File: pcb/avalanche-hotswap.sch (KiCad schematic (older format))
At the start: 107 parts, among them J1 TRRS, J2 LED, J3 OLED, P1 i2c_pin, P2 i2c_pin, SW1 SW_Push, SW10 SW_Push, SW11 SW_Push, SW12 SW_Push, SW13 SW_Push, SW14 SW_Push, SW15 SW_Push, SW16 SW_Push, SW17 SW_Push, SW18 SW_Push, SW19 SW_Push, SW2 SW_Push, SW20 SW_Push, SW21 SW_Push, SW22 SW_Push, SW23 SW_Push, SW24 SW_Push, SW25 SW_Push, SW26 SW_Push, SW27 SW_Push, SW28 SW_Push, SW29 SW_Push, SW3 SW_Push, SW30 SW_Push, SW31 SW_Push, SW32 SW_Push, SW4 SW_Push, SW5 SW_Push, SW6 SW_Push, SW7 SW_Push, SW8 SW_Push, SW9 SW_Push, U1 ProMicro

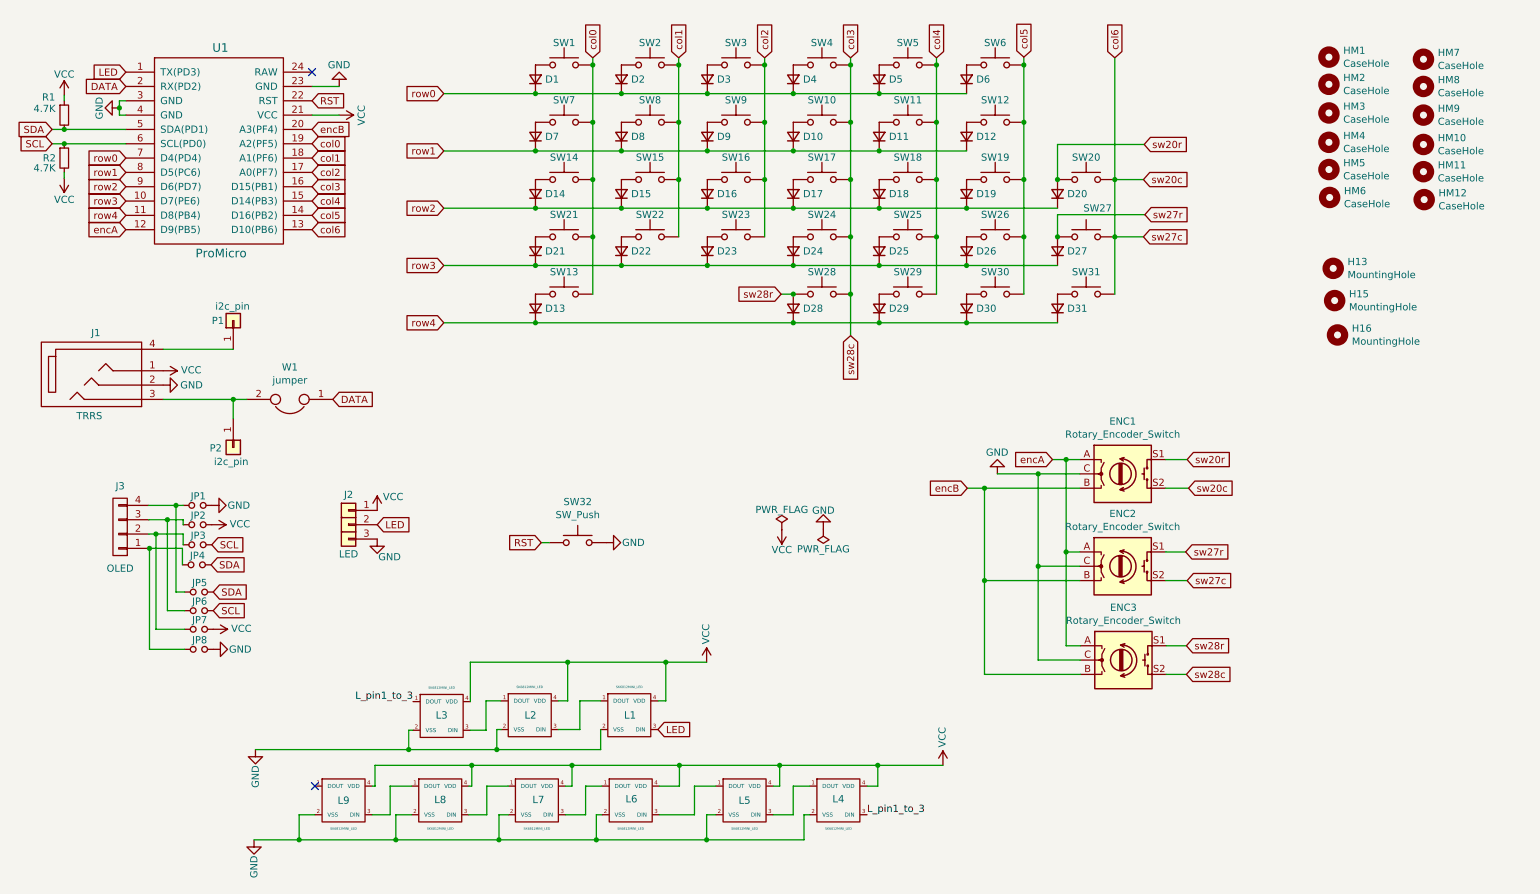
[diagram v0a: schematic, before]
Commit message: WIP on smd diodes...
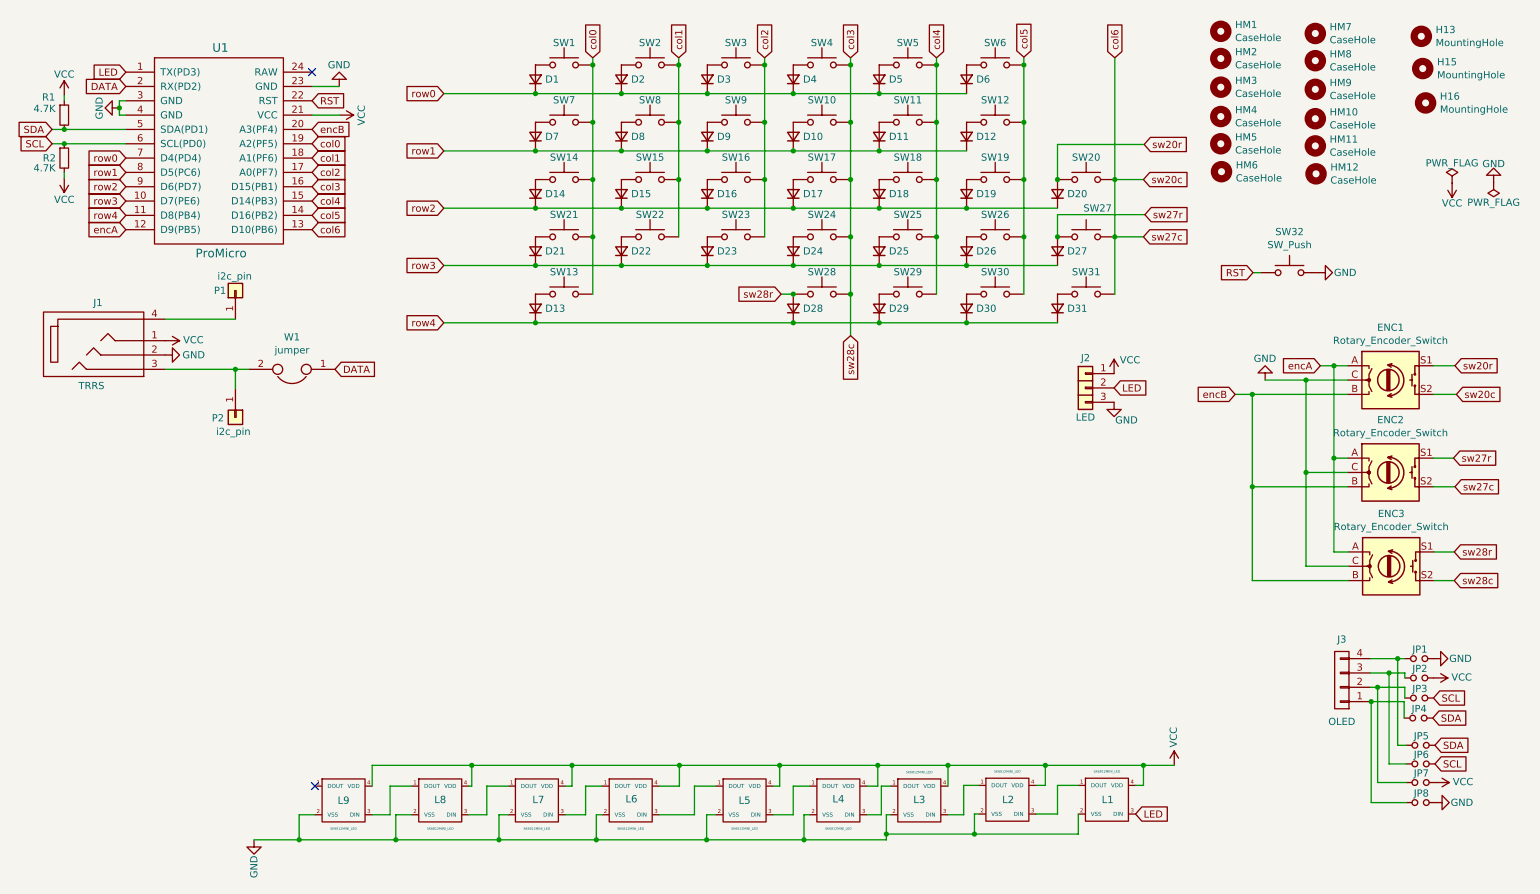
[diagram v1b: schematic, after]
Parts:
- D10, D11, D12, D8, D9: footprint used_footprints:D3_TH_SMD -> used_footprints:diode_SMD
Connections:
- net L_pin1_to_3: no longer names the net of L3.1 (DOUT), L4.3 (DIN)
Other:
- moved on the sheet: ENC1, ENC2, ENC3, H13, H15, H16, HM1, HM10, HM11, HM12, HM2, HM3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

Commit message: WIP on diodes. Moved a case hole a little bit
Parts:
- D13, D14, D15, D16, D17, D18, D19, D20: footprint used_footprints:D3_TH_SMD -> used_footprints:diode_SMD
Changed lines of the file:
@@
 F 0 "D13" V 4145 2522 50  0000 R CNN
 F 1 "1N4148" V 4100 2522 50  0001 R CNN
-F 2 "used_footprints:D3_TH_SMD" V 4145 2590 50  0001 C CNN
+F 2 "used_footprints:diode_SMD" V 4145 2590 50  0001 C CNN
 F 3 "~" V 4145 2590 50  0001 C CNN
 	1    4145 2590
-	0    -1   -1   0
-$EndComp
-$Comp
-L Device:D_Small D14
-U 1 1 5DAD50E5
-P 4145 1790
-F 0 "D14" V 4145 1722 50  0000 R CNN
-F 1 "1N4148" V 4100 1722 50  0001 R CNN
-F 2 "used_footprints:D3_TH_SMD" V 4145 1790 50  0001 C CNN
-F 3 "~" V 4145 1790 50  0001 C CNN
-	1    4145 1790
 	0    -1   -1   0
 $EndComp
@@
 F 0 "D15" V 4745 1722 50  0000 R CNN
 F 1 "1N4148" V 4700 1722 50  0001 R CNN
-F 2 "used_footprints:D3_TH_SMD" V 4745 1790 50  0001 C CNN
+F 2 "used_footprints:diode_SMD" V 4745 1790 50  0001 C CNN
 F 3 "~" V 4745 1790 50  0001 C CNN
 	1    4745 1790
@@
 F 0 "D16" V 5345 1722 50  0000 R CNN
 F 1 "1N4148" V 5300 1722 50  0001 R CNN
-F 2 "used_footprints:D3_TH_SMD" V 5345 1790 50  0001 C CNN
+F 2 "used_footprints:diode_SMD" V 5345 1790 50  0001 C CNN
 F 3 "~" V 5345 1790 50  0001 C CNN
 	1    5345 1790
@@
 F 0 "D17" V 5945 1722 50  0000 R CNN
 F 1 "1N4148" V 5900 1722 50  0001 R CNN
-F 2 "used_footprints:D3_TH_SMD" V 5945 1790 50  0001 C CNN
+F 2 "used_footprints:diode_SMD" V 5945 1790 50  0001 C CNN
 F 3 "~" V 5945 1790 50  0001 C CNN
 	1    5945 1790
@@
 F 0 "D18" V 6545 1722 50  0000 R CNN
 F 1 "1N4148" V 6500 1722 50  0001 R CNN
-F 2 "used_footprints:D3_TH_SMD" V 6545 1790 50  0001 C CNN
+F 2 "used_footprints:diode_SMD" V 6545 1790 50  0001 C CNN
 F 3 "~" V 6545 1790 50  0001 C CNN
 	1    6545 1790
@@
 Wire Wire Line
 	5945 2290 6545 2290
-Connection ~ 4145 1890
-Wire Wire Line
-	4145 1890 4745 1890
 Connection ~ 4745 1890
 Wire Wire Line
@@
 F 0 "D19" V 7155 1722 50  0000 R CNN
 F 1 "1N4148" V 7110 1722 50  0001 R CNN
-F 2 "used_footprints:D3_TH_SMD" V 7155 1790 50  0001 C CNN
+F 2 "used_footprints:diode_SMD" V 7155 1790 50  0001 C CNN
 F 3 "~" V 7155 1790 50  0001 C CNN
 	1    7155 1790
@@
 F 0 "D20" V 7790 1722 50  0000 R CNN
 F 1 "1N4148" V 7745 1722 50  0001 R CNN
-F 2 "used_footprints:D3_TH_SMD" V 7790 1790 50  0001 C CNN
+F 2 "used_footprints:diode_SMD" V 7790 1790 50  0001 C CNN
 F 3 "~" V 7790 1790 50  0001 C CNN
 	1    7790 1790
@@
 	9150 4490 9820 4490
 Connection ~ 4145 2690
-Wire Wire Line
-	3505 1890 4145 1890
 Wire Wire Line
 	4545 2090 4545 2490
@@
 Connection ~ 7025 5780
 Connection ~ 6535 5780
+Wire Wire Line
+	3505 1890 4145 1890
+Wire Wire Line
+	4145 1890 4745 1890
+Connection ~ 4145 1890
+$Comp
+L Device:D_Small D14
+U 1 1 5DAD50E5
+P 4145 1790
+F 0 "D14" V 4145 1722 50  0000 R CNN
+F 1 "1N4148" V 4100 1722 50  0001 R CNN
+F 2 "used_footprints:diode_SMD" V 4145 1790 50  0001 C CNN
+F 3 "~" V 4145 1790 50  0001 C CNN
+	1    4145 1790
+	0    -1   -1   0
+$EndComp
 $EndSCHEMATC
